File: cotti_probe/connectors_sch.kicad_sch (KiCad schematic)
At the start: 60 parts, among them J2 Conn_01x10, J3 Conn_01x10, J4 Conn_01x05, J5 Conn_01x05, J6 Conn_01x05, J7 Conn_01x05, J8 Conn_01x02, J9 Conn_01x02, Q1 PMOS Kp=0.2 |Vth|=0.8, U5 74HC595, U6 74LV1T125GWH

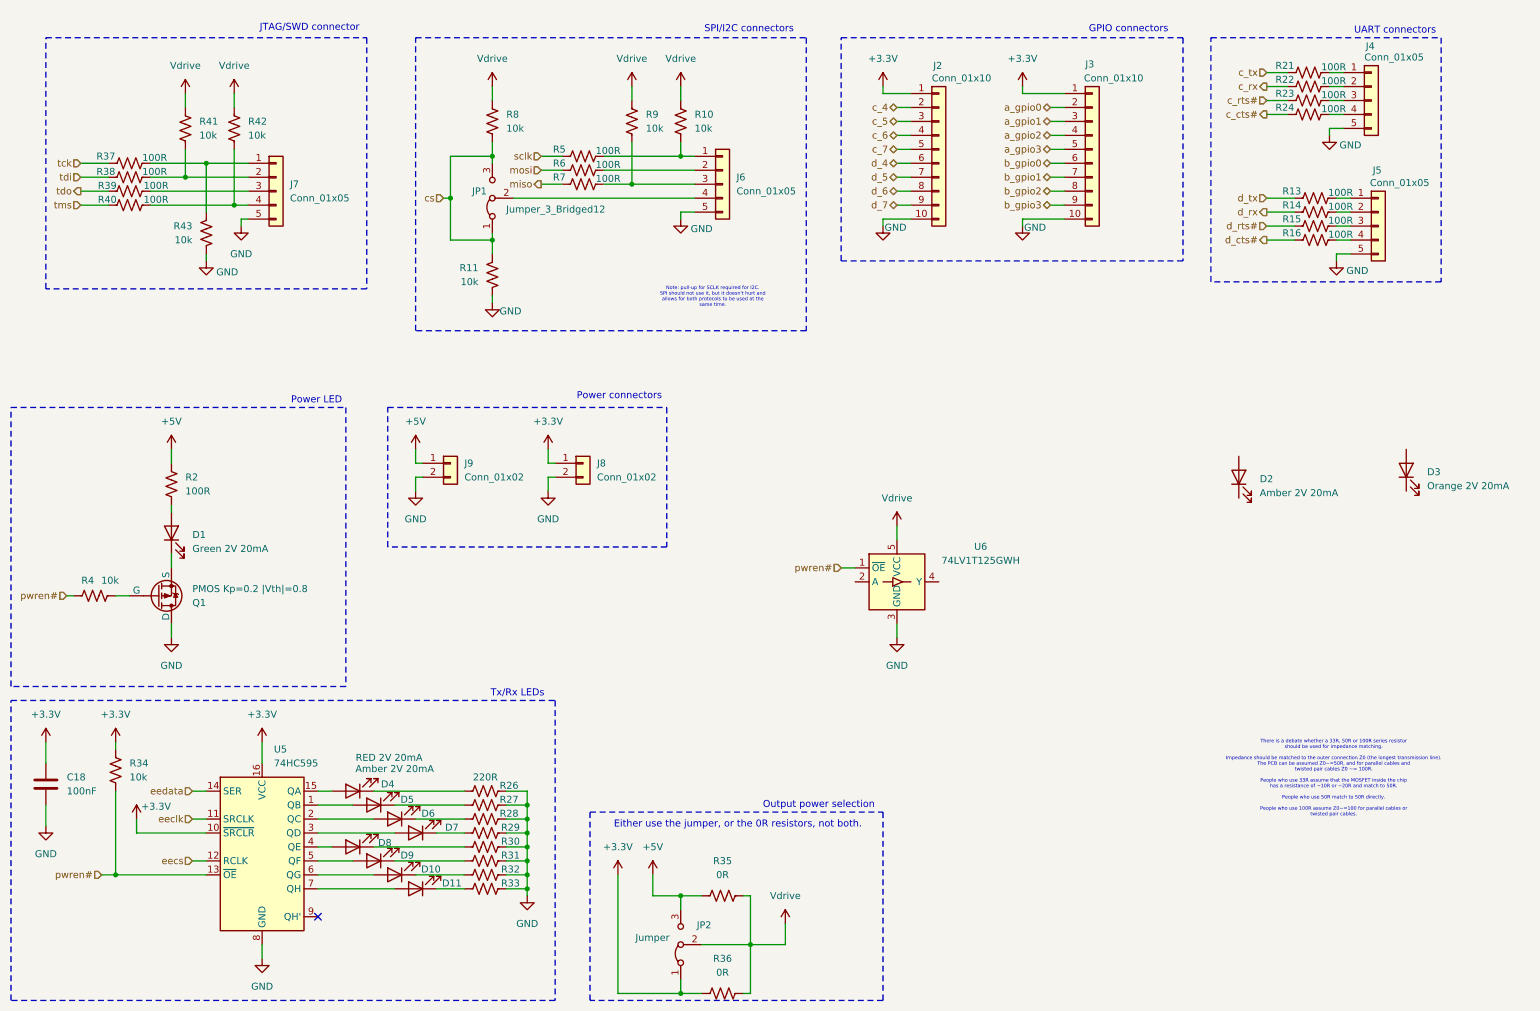
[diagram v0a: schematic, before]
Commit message: feat: gerbers for cotti probe
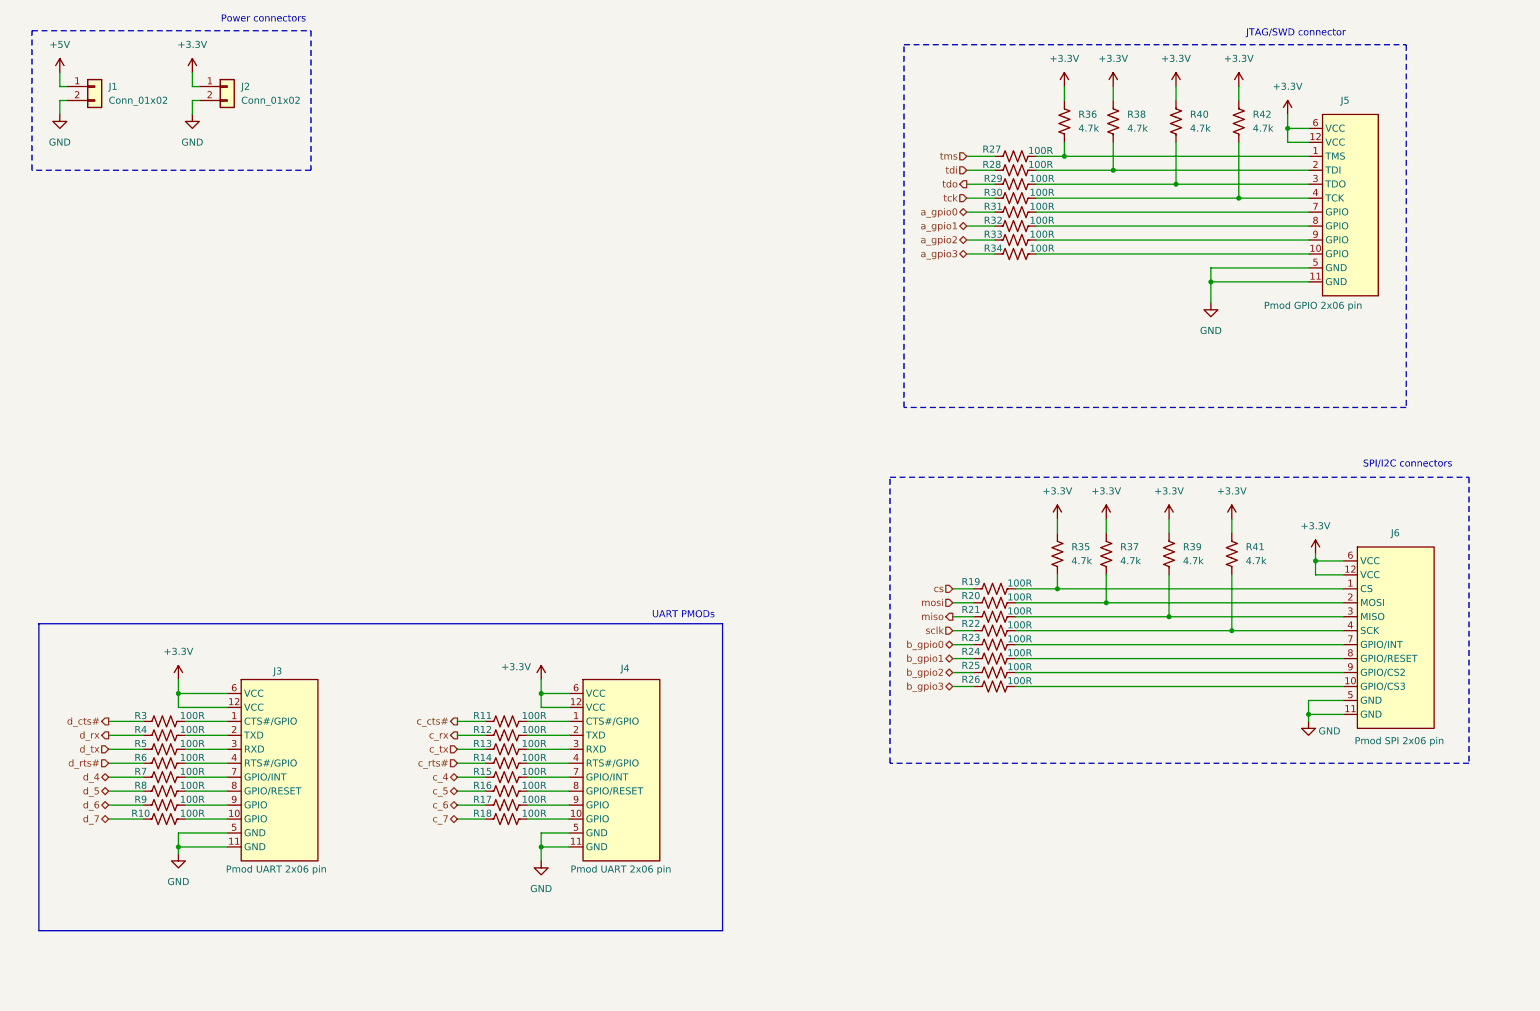
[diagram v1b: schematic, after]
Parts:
- removed C18: 100nF, symbol Device:C
- removed D1: Green 2V 20mA, symbol Device:LED
- removed D10, D4, D6, D8: RED 2V 20mA, symbol Device:LED
- removed D11, D2, D5, D7, D9: Amber 2V 20mA, symbol Device:LED
- removed D3: Orange 2V 20mA, symbol Device:LED
- removed J2, J3: Conn_01x10, symbol Connector_Generic:Conn_01x10
- removed J4, J5, J6, J7: Conn_01x05, symbol Connector_Generic:Conn_01x05
- removed JP1: Jumper_3_Bridged12, symbol Jumper:Jumper_3_Bridged12
- removed JP2: Jumper, symbol Jumper:Jumper_3_Bridged12
- removed Q1: PMOS Kp=0.2 |Vth|=0.8, symbol Simulation_SPICE:PMOS
- removed R2, R21: 100R, symbol Device:R_US
- removed R27, R28, R29, R30: 220R, symbol Device:R_US
- removed R36: 0R, symbol Device:R_US
- removed R43: 10k, symbol Device:R_US
- removed U5: 74HC595, symbol 74xx:74HC595
- removed U6: 74LV1T125GWH, Package_TO_SOT_SMD:SOT-23-5, symbol Logic_LevelTranslator:SN74LV1T125DBV
- added J3, J4: Pmod UART 2x06 pin, cotti_footprints:Pmod_2x06_pin, symbol cotti_pmod:pmod_uart_2x06_pin
- added J5: Pmod GPIO 2x06 pin, cotti_footprints:Pmod_2x06_pin, symbol cotti_pmod:pmod_jtag_2x06_pin
- added J6: Pmod SPI 2x06 pin, cotti_footprints:Pmod_2x06_pin, symbol cotti_pmod:pmod_spi_2x06_pin
- added R12, R17, R18, R25, R3, R5, R6, R7: 100R, Resistor_SMD:R_0805_2012Metric_Pad1.20x1.40mm_HandSolder, symbol Device:R_US
- added R37, R39, R40, R41, R42: 4.7k, Resistor_SMD:R_0805_2012Metric_Pad1.20x1.40mm_HandSolder, symbol Device:R_US
- J1: renamed from J9; footprint (none) -> Connector_PinHeader_2.54mm:PinHeader_1x02_P2.54mm_Vertical; now left out of the parts list
- J2: renamed from J8; footprint (none) -> Connector_PinHeader_2.54mm:PinHeader_1x02_P2.54mm_Vertical; now left out of the parts list
- R10, R11, R34, R4, R8, R9: value 10k -> 100R; footprint (none) -> Resistor_SMD:R_0805_2012Metric_Pad1.20x1.40mm_HandSolder; Digikey (none) -> https://www.digikey.com/en/products/detail/yageo/RC0805FR-1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; Mfr. (none) -> YAGEO; Mfr. P/N (none) -> RC0805FR-10100RL
- R13, R14, R15, R16, R22, R23, R24: footprint (none) -> Resistor_SMD:R_0805_2012Metric_Pad1.20x1.40mm_HandSolder; Digikey (none) -> https://www.digikey.com/en/products/detail/yageo/RC0805FR-1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; Mfr. (none) -> YAGEO; Mfr. P/N (none) -> RC0805FR-10100RL
- R19: renamed from R5; footprint (none) -> Resistor_SMD:R_0805_2012Metric_Pad1.20x1.40mm_HandSolder; Digikey (none) -> https://www.digikey.com/en/products/detail/yageo/RC0805FR-1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; Mfr. (none) -> YAGEO; Mfr. P/N (none) -> RC0805FR-10100RL
- R20: renamed from R6; footprint (none) -> Resistor_SMD:R_0805_2012Metric_Pad1.20x1.40mm_HandSolder; Digikey (none) -> https://www.digikey.com/en/products/detail/yageo/RC0805FR-1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; Mfr. (none) -> YAGEO; Mfr. P/N (none) -> RC0805FR-10100RL
- R21: renamed from R7; footprint (none) -> Resistor_SMD:R_0805_2012Metric_Pad1.20x1.40mm_HandSolder; Digikey (none) -> https://www.digikey.com/en/products/detail/yageo/RC0805FR-1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; Mfr. (none) -> YAGEO; Mfr. P/N (none) -> RC0805FR-10100RL
- R26, R31, R32, R33: value 220R -> 100R; footprint (none) -> Resistor_SMD:R_0805_2012Metric_Pad1.20x1.40mm_HandSolder; Digikey (none) -> https://www.digikey.com/en/products/detail/yageo/RC0805FR-1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; Mfr. (none) -> YAGEO; Mfr. P/N (none) -> RC0805FR-10100RL
- R27: renamed from R37; footprint (none) -> Resistor_SMD:R_0805_2012Metric_Pad1.20x1.40mm_HandSolder; Digikey (none) -> https://www.digikey.com/en/products/detail/yageo/RC0805FR-1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; Mfr. (none) -> YAGEO; Mfr. P/N (none) -> RC0805FR-10100RL
- R28: renamed from R38; footprint (none) -> Resistor_SMD:R_0805_2012Metric_Pad1.20x1.40mm_HandSolder; Digikey (none) -> https://www.digikey.com/en/products/detail/yageo/RC0805FR-1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; Mfr. (none) -> YAGEO; Mfr. P/N (none) -> RC0805FR-10100RL
- R29: renamed from R39; footprint (none) -> Resistor_SMD:R_0805_2012Metric_Pad1.20x1.40mm_HandSolder; Digikey (none) -> https://www.digikey.com/en/products/detail/yageo/RC0805FR-1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; Mfr. (none) -> YAGEO; Mfr. P/N (none) -> RC0805FR-10100RL
- R30: renamed from R40; footprint (none) -> Resistor_SMD:R_0805_2012Metric_Pad1.20x1.40mm_HandSolder; Digikey (none) -> https://www.digikey.com/en/products/detail/yageo/RC0805FR-1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; Mfr. (none) -> YAGEO; Mfr. P/N (none) -> RC0805FR-10100RL
- R35: value 0R -> 4.7k; footprint (none) -> Resistor_SMD:R_0805_2012Metric_Pad1.20x1.40mm_HandSolder; Digikey (none) -> https://www.digikey.com/en/products/detail/yageo/RC0805FR-1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; Mfr. (none) -> YAGEO; Mfr. P/N (none) -> RC0805FR-134K7L
- R36: renamed from R41; value 10k -> 4.7k; footprint (none) -> Resistor_SMD:R_0805_2012Metric_Pad1.20x1.40mm_HandSolder; Digikey (none) -> https://www.digikey.com/en/products/detail/yageo/RC0805FR-1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; Mfr. (none) -> YAGEO; Mfr. P/N (none) -> RC0805FR-134K7L
- R38: renamed from R42; value 10k -> 4.7k; footprint (none) -> Resistor_SMD:R_0805_2012Metric_Pad1.20x1.40mm_HandSolder; Digikey (none) -> https://www.digikey.com/en/products/detail/yageo/RC0805FR-1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; Mfr. (none) -> YAGEO; Mfr. P/N (none) -> RC0805FR-134K7L
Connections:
- net +3.3V: now also R35.1, R36.1, R38.1, J3.12 (VCC), J3.6 (VCC), J4.12 (VCC), J4.6 (VCC), J5.12 (VCC), J5.6 (VCC), J6.12 (VCC), J6.6 (VCC), R37.1, R39.1, R40.1, R41.1, R42.1; no longer R34.1
- net +5V: no longer R35.1
- net GND: now also J3.11 (GND), J3.5 (GND), J4.11 (GND), J4.5 (GND), J5.11 (GND), J5.5 (GND), J6.11 (GND), J6.5 (GND); no longer R11.1, R26.2, R31.2, R32.2, R33.2
- net a_gpio0: now also R31.1
- net a_gpio1: now also R32.1
- net a_gpio2: now also R33.1
- net a_gpio3: now also R34.1
- net b_gpio0: now also R23.1
- net b_gpio1: now also R24.1
- net b_gpio2: now also R25.1
- net b_gpio3: now also R26.1
- net c_4: now also R15.1
- net c_5: now also R16.1
- net c_6: now also R17.1
- net c_7: now also R18.1
- net c_cts#: now also R11.1; no longer R24.1
- net c_rts#: now also R14.1; no longer R23.1
- net c_rx: now also R12.1; no longer R22.1
- net c_tx: now also R13.1
- net cs: now also R19.1; no longer R11.2, R8.2
- net d_4: now also R7.1
- net d_5: now also R8.1
- net d_6: now also R9.1
- net d_7: now also R10.1
- net d_cts#: now also R3.1; no longer R16.1
- net d_rts#: now also R6.1; no longer R15.1
- net d_rx: now also R4.1; no longer R14.1
- net d_tx: now also R5.1; no longer R13.1
- net sclk: now also R22.1; no longer R19.1
- net tck: now also R30.1; no longer R27.1
- net tms: now also R27.1; no longer R30.1
- net at R19.2: now also R35.2, J6.1 (CS); no longer R10.2
- net at R22.2: now also J6.4 (SCK), R41.2
- net at R23.2: now also J6.7 (GPIO/INT)
- net at R24.2: now also J6.8 (GPIO/RESET)
- net at R16.2: now also J4.8 (GPIO/RESET)
- net at R27.2: now also R36.2, J5.1 (TMS)
- net at R28.2: now also R38.2, J5.2 (TDI); no longer R36.2
- net at R29.2: now also J5.3 (TDO), R40.2
- net at R30.2: now also J5.4 (TCK), R42.2; no longer R38.2
- net at R4.2: now also J3.2 (TXD)
- net at R13.2: now also J4.3 (RXD)
- net at R14.2: now also J4.4 (RTS#/GPIO)
- net at R15.2: now also J4.7 (GPIO/INT)
- net at R21.2: now also J6.3 (MISO), R39.2; no longer R9.2
- net at R20.2: now also J6.2 (MOSI), R37.2
- removed net Vdrive: R10.1, R35.2, R36.1, R38.1, R8.1, R9.1
- net pwren#: no longer names the net of R34.2
- net pwren#: now also J5.10 (GPIO); no longer R4.1
- new net: J5.7 (GPIO), R31.2
- new net: J5.8 (GPIO), R32.2
- new net: J5.9 (GPIO), R33.2
- new net: J4.9 (GPIO), R17.2
- new net: J4.10 (GPIO), R18.2
- new net: J4.2 (TXD), R12.2
- new net: J6.9 (GPIO/CS2), R25.2
- new net: J3.3 (RXD), R5.2
- new net: J3.8 (GPIO/RESET), R8.2
- new net: J6.10 (GPIO/CS3), R26.2
- new net: J4.1 (CTS#/GPIO), R11.2
- new net: J3.9 (GPIO), R9.2
- new net: J3.7 (GPIO/INT), R7.2
- new net: J3.1 (CTS#/GPIO), R3.2
- new net: J3.10 (GPIO), R10.2
- new net: J3.4 (RTS#/GPIO), R6.2
- no-connect marks 1 -> 0
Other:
- note added: "UART PMODs"
- note removed: "Either use the jumper, or the 0R resistors, not both."
- note removed: "GPIO connectors"
- note removed: "Note: pull-up for SCLK required for I2C. SPI should not use it, but it doesn't hurt and allows for both protocols to be used at the same time."
- note removed: "Output power selection"
- note removed: "Power LED"
- note removed: "There is a debate whether a 33R, 50R or 100R series resistor should be used for impedance matching. Impedance should be matched to the outer connection Z0 (the longest transmission line). The PCB can be assumed Z0~=50R, and for parallel cables and twisted pair cables Z0 ~= 100R. People who use 33R assume that the MOSFET inside the chip has a resistance of ~10R or ~20R and match to 50R. People who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"
- note removed: "Tx/Rx LEDs"
- note removed: "UART connectors"
- moved on the sheet: J1, J2, R19, R20, R21, R27, R28, R29, R30, R36, R38
